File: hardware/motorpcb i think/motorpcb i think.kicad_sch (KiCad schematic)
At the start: 1 part, among them U1 PCA9685PW_Q900_118

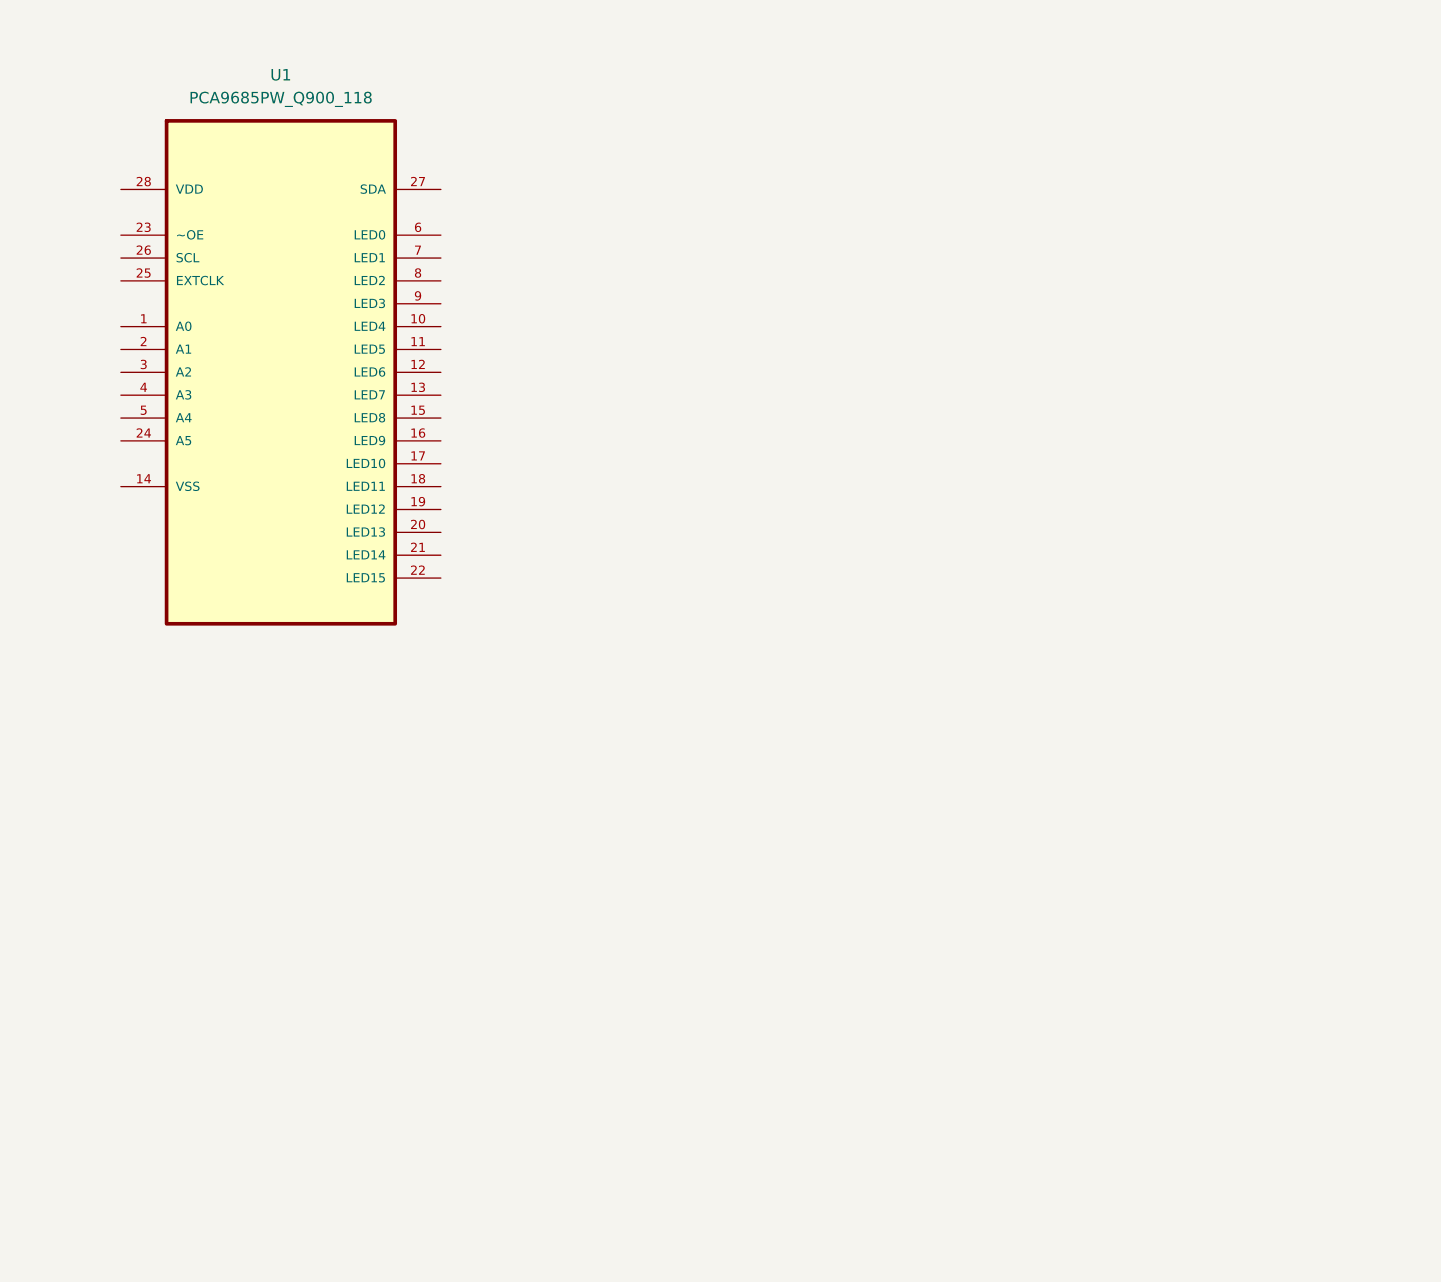
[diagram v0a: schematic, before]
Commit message: continued schematic work
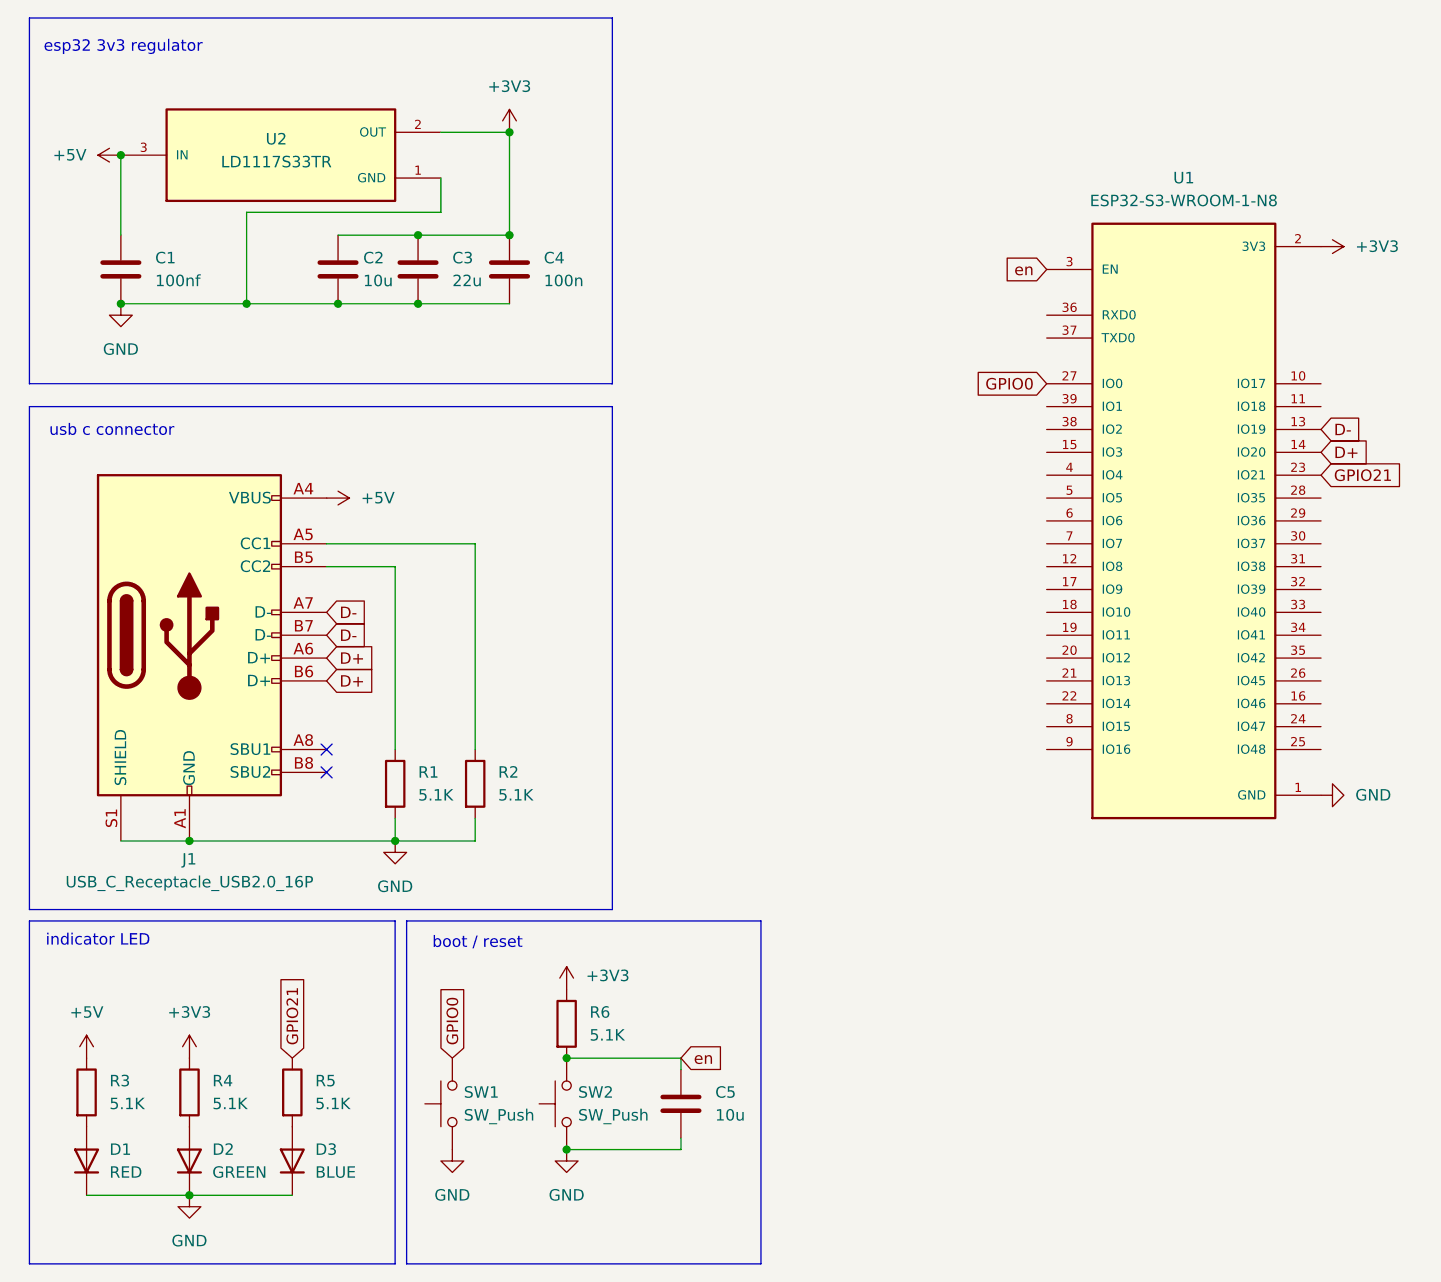
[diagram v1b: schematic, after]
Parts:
- removed U1: PCA9685PW_Q900_118, symbol motorpcb i think:PCA9685PW_Q900_118
- added C1: 100nf, symbol Device:C
- added C2, C5: 10u, symbol Device:C
- added C3: 22u, symbol Device:C
- added C4: 100n, symbol Device:C
- added D1: RED, symbol Device:D
- added D2: GREEN, symbol Device:D
- added D3: BLUE, symbol Device:D
- added J1: USB_C_Receptacle_USB2.0_16P, symbol Connector:USB_C_Receptacle_USB2.0_16P
- added R1, R2, R3, R4, R5, R6: 5.1K, symbol Device:R
- added SW1, SW2: SW_Push, symbol Switch:SW_Push
- added U1: ESP32-S3-WROOM-1-N8, ESP32-S3-WROOM-1-N8:XCVR_ESP32-S3-WROOM-1-N8, symbol motorpcb i think:ESP32-S3-WROOM-1-N8
- added U2: LD1117S33TR, LD1117S33TR:SOT230P700X180-4N, symbol motorpcb i think:LD1117S33TR
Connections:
- new net: J1.A5 (CC1), R2.1
- new net: D1.2 (A), R3.2
- new net: J1.B5 (CC2), R1.1
- new net: D3.2 (A), R5.2
- new net: D2.2 (A), R4.2
- new net +3V3: C2.1, C3.1, C4.1, R4.1, R6.1, U1.2 (3V3), U2.2 (OUT), U2.4 (OUT)
- new net +5V: C1.1, J1.A4 (VBUS), J1.A9 (VBUS), J1.B4 (VBUS), J1.B9 (VBUS), R3.1, U2.3 (IN)
- new net D+: J1.A6 (D+), J1.B6 (D+), U1.14 (IO20)
- new net D-: J1.A7 (D-), J1.B7 (D-), U1.13 (IO19)
- new net GND: C1.2, C2.2, C3.2, C4.2, C5.2, D1.1 (K), D2.1 (K), D3.1 (K), J1.A1 (GND), J1.A12 (GND), J1.B1 (GND), J1.B12 (GND), J1.S1 (SHIELD), R1.2, R2.2, SW1.1, SW2.1, U1.1 (GND), U1.40 (GND), U1.41_1 (GND), U1.41_2 (GND), U1.41_3 (GND), U1.41_4 (GND), U1.41_5 (GND), U1.41_6 (GND), U1.41_7 (GND), U1.41_8 (GND), U1.41_9 (GND), U2.1 (GND)
- new net GPIO0: SW1.2, U1.27 (IO0)
- new net GPIO21: R5.1, U1.23 (IO21)
- new net en: C5.1, R6.2, SW2.2, U1.3 (EN)
- no-connect marks 0 -> 2
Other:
- note added: "boot / reset"
- note added: "esp32 3v3 regulator"
- note added: "indicator LED"
- note added: "usb c connector"
